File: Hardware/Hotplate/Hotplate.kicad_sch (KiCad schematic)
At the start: 23 parts, among them J4 Conn_01x01_Pin, J5 Conn_01x01_Pin, Q2 Q_NMOS_GDS, SW1 SW_Push, SW2 SW_Push, SW3 SW_Push, SW4 SW_Push, U1 STM32F301K6Tx

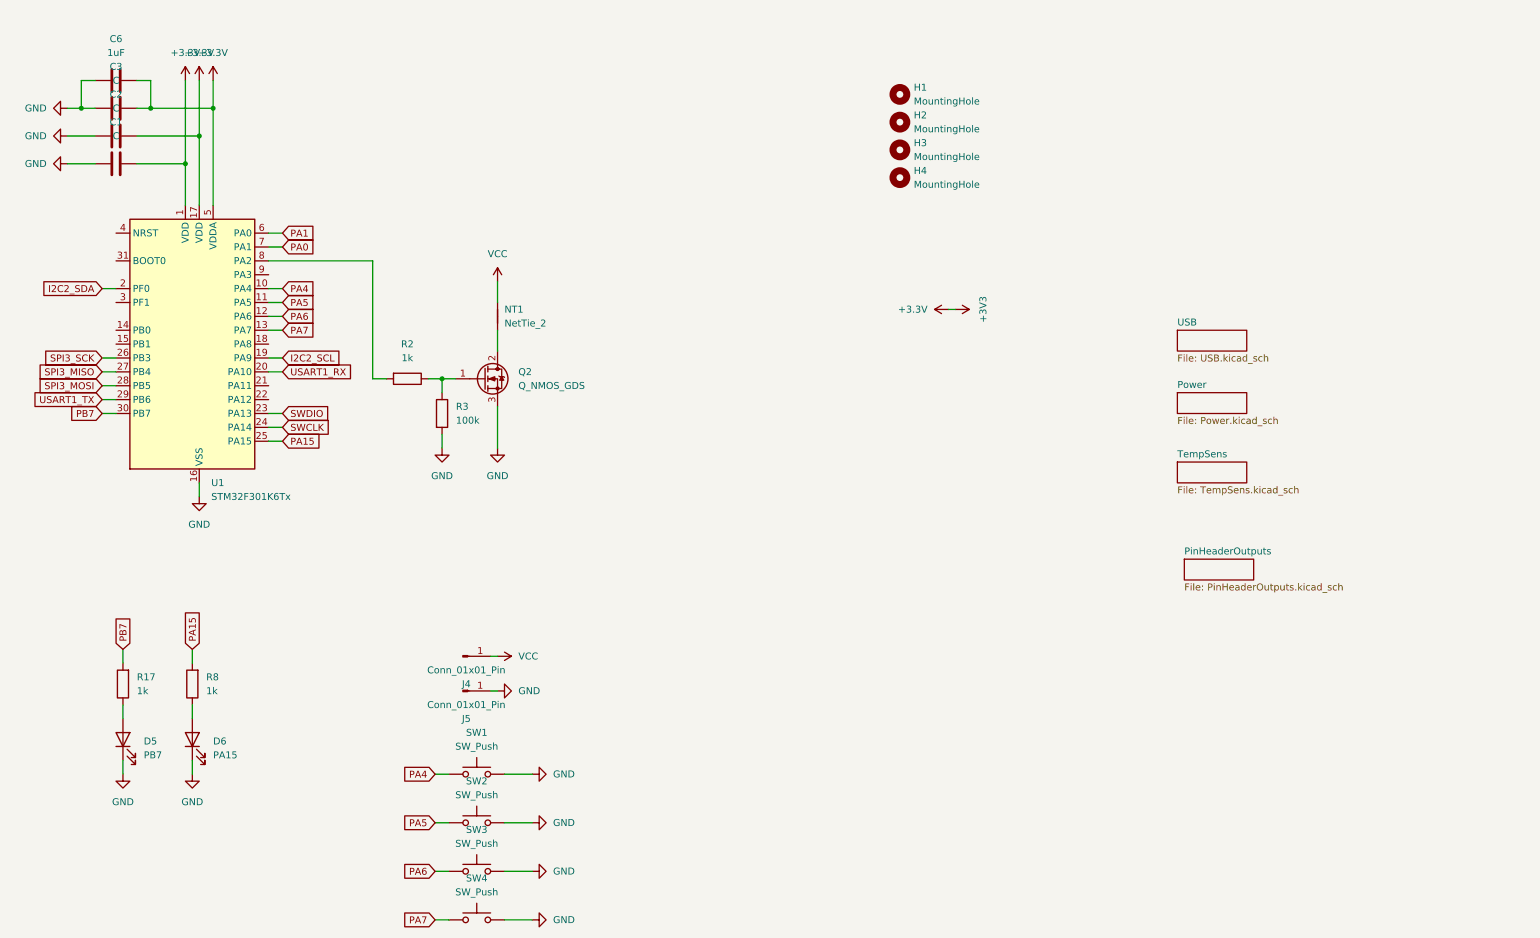
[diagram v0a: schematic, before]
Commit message: V2
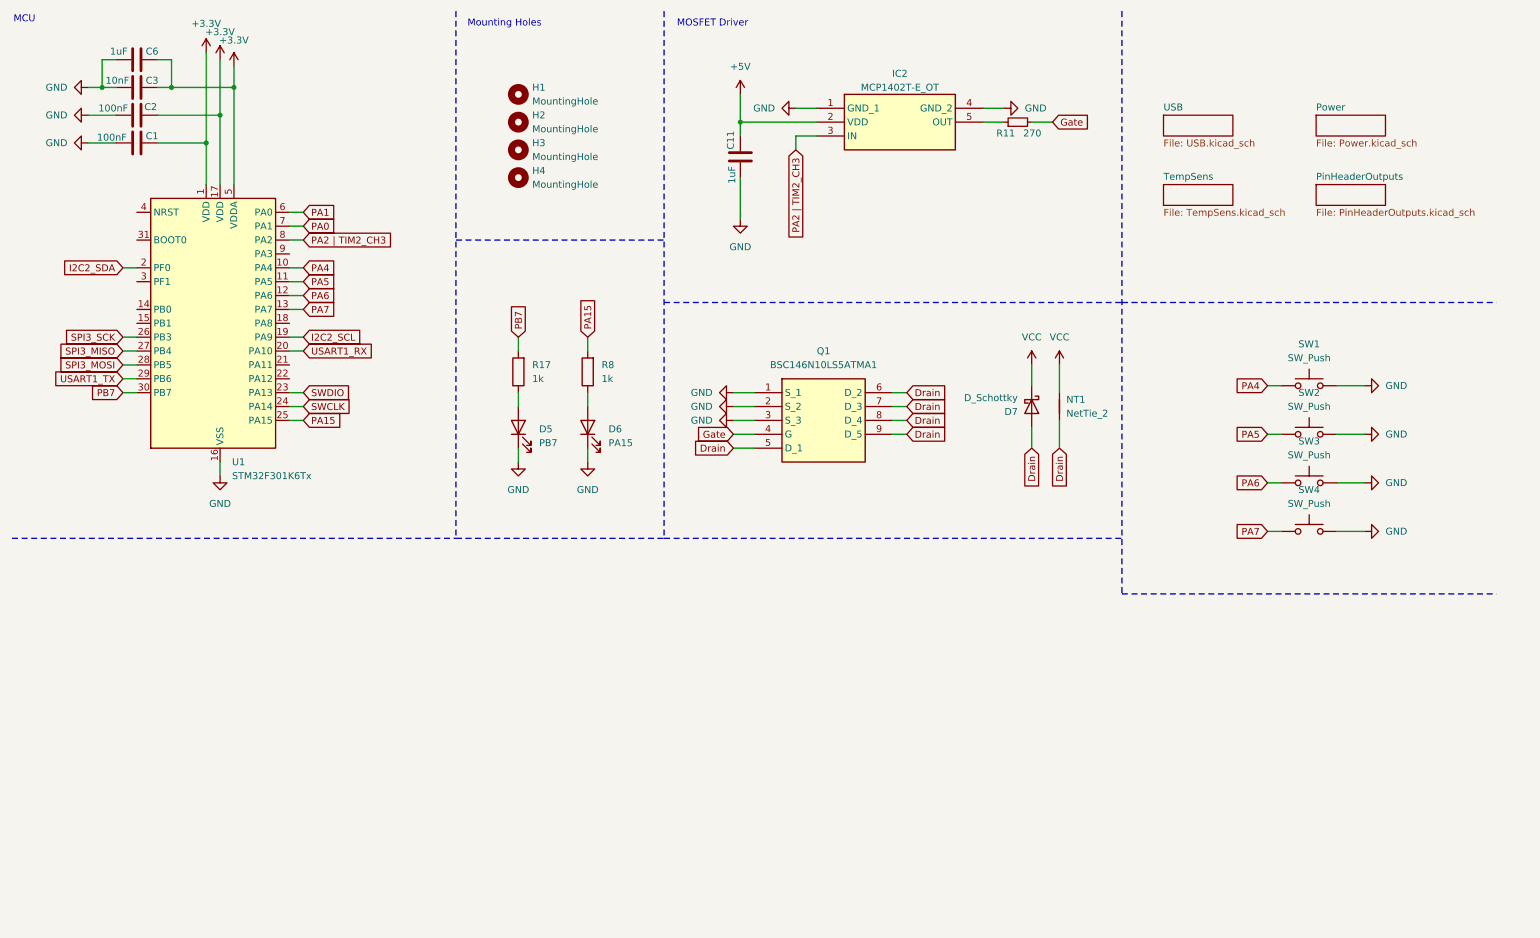
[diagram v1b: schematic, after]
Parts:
- removed J4, J5: Conn_01x01_Pin, Connector_Wire:SolderWire-1.5sqmm_1x01_D1.7mm_OD3mm, symbol Connector:Conn_01x01_Pin
- removed Q2: Q_NMOS_GDS, Package_TO_SOT_SMD:TO-252-2, symbol Device:Q_NMOS_GDS
- removed R2: 1k, Resistor_SMD:R_0805_2012Metric, symbol Device:R
- removed R3: 100k, Resistor_SMD:R_0805_2012Metric, symbol Device:R
- added C11: 1uF, Capacitor_SMD:C_0603_1608Metric, symbol Device:C
- added D7: D_Schottky, Diode_THT:D_DO-15_P10.16mm_Horizontal, symbol Device:D_Schottky
- added IC2: MCP1402T-E_OT, SOT95P270X145-5N, symbol SamacSys_Parts:MCP1402T-E_OT
- added Q1: BSC146N10LS5ATMA1, SamacSys_Parts:BSC146N10LS5ATMA1, symbol SamacSys_Parts:BSC146N10LS5ATMA1
- added R11: 270, Resistor_SMD:R_0603_1608Metric_Pad0.98x0.95mm_HandSolder, symbol Device:R_Small
- C1, C2: value C -> 100nF
- C3: value C -> 10nF
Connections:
- net GND: now also C11.1, IC2.1 (GND_1), IC2.4 (GND_2), Q1.1 (S_1), Q1.2 (S_2), Q1.3 (S_3)
- net VCC: now also D7.1 (K)
- net Drain: now reaches NT1.1
- net Drain: now also D7.2 (A), Q1.5 (D_1), Q1.6 (D_2), Q1.7 (D_3), Q1.8 (D_4), Q1.9 (D_5)
- net PA2 | TIM2_CH3: now reaches U1.8 (PA2)
- net PA2 | TIM2_CH3: now also IC2.3 (IN)
- new net: IC2.5 (OUT), R11.1
- new net +5V: C11.2, IC2.2 (VDD)
- new net Gate: Q1.4 (G), R11.2
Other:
- note added: "MCU"
- note added: "MOSFET Driver"
- note added: "Mounting Holes"
- moved on the sheet: C1, C2, C3, C6, D5, D6, H1, H2, H3, H4, NT1, R17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
